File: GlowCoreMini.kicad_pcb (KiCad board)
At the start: 2 copper layers, 66 x 26.7 mm, 34 parts, among them J2 DC-042C-Z-2.5-A, J3 Conn_02x06_Counter_Clockwise, J4 WJ500V-5.08-3P, Q1 SK338P, Q2 MMBT2222A, Q3 MMBT2222A, SW1 TS-1185EC-C-D-B, U1 SN74AHCT32QPWRQ1, U2 ESP32-WROOM-32E (4MB), U3 BL1117-33CX, U4 CP2104

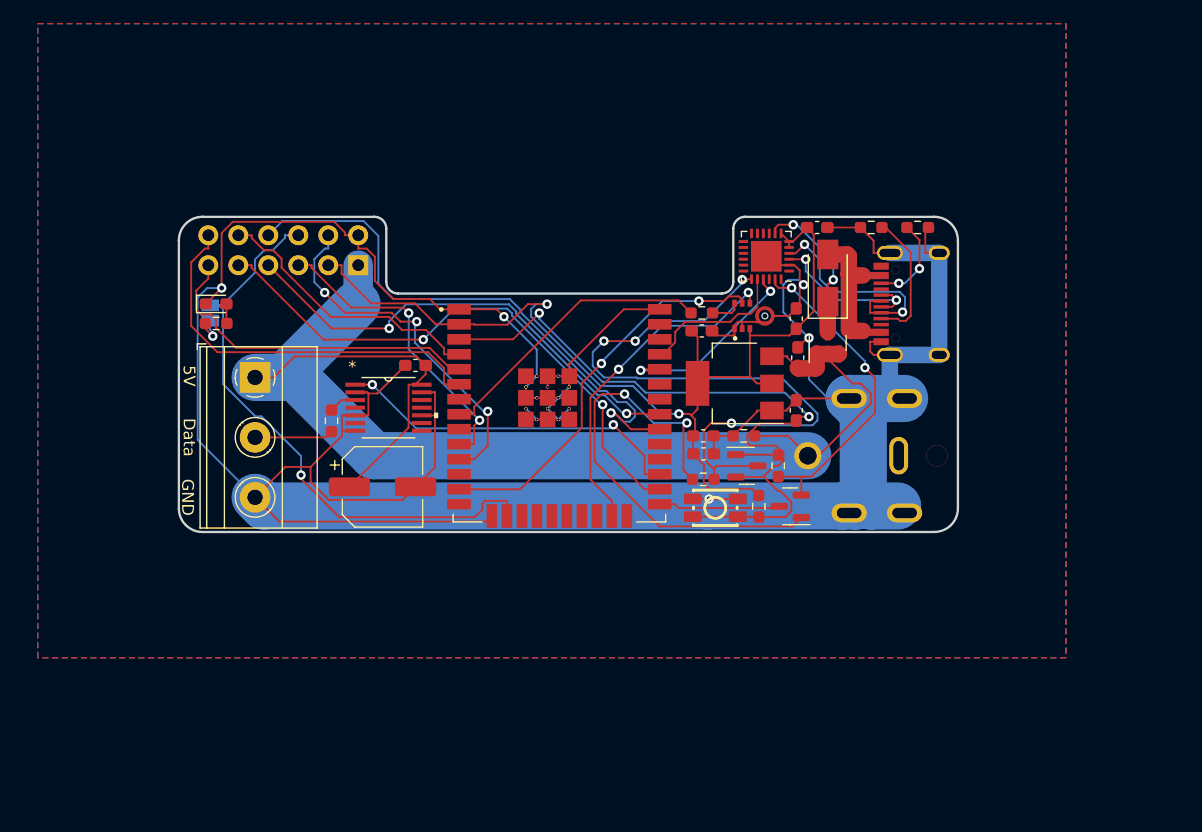
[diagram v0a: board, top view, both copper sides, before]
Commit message: updated pcb design (still in dev)
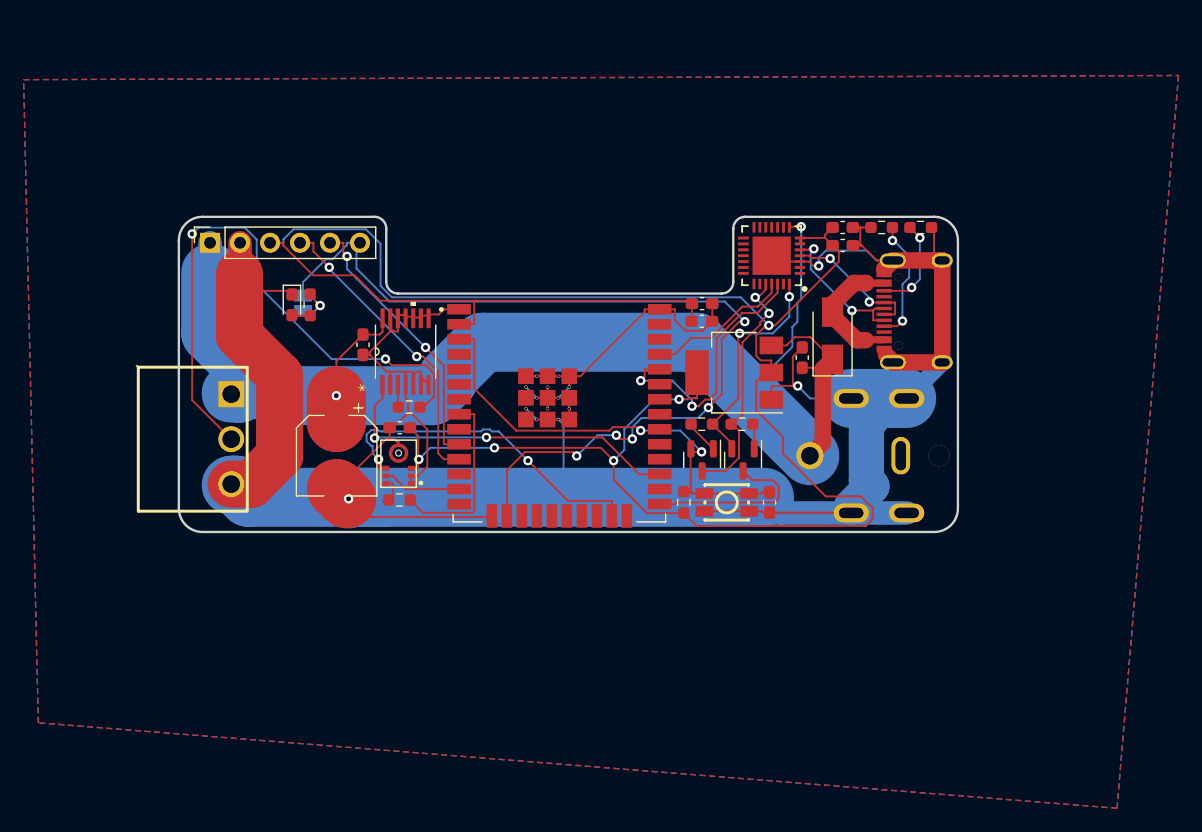
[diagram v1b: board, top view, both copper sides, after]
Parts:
- removed C5: 1uF, Capacitor_SMD:C_0603_1608Metric_Pad1.08x0.95mm_HandSolder
- removed J3: Conn_02x06_Counter_Clockwise, Connector_PinSocket_2.54mm:PinSocket_2x06_P2.54mm_Vertical
- removed J4: WJ500V-5.08-3P, TerminalBlock_Phoenix:TerminalBlock_Phoenix_MKDS-1,5-3-5.08_1x03_P5.08mm_Horizontal
- removed Q1: SK338P, Package_TO_SOT_SMD:SOT-23
- removed R2: 100K, Resistor_SMD:R_0603_1608Metric_Pad0.98x0.95mm_HandSolder
- added C10: 0.1uF, Capacitor_SMD:C_0603_1608Metric_Pad1.08x0.95mm_HandSolder, F.Cu at (163.3, 84.3)
- added J1: Conn_01x06, Connector_PinSocket_2.54mm:PinSocket_1x06_P2.54mm_Vertical, F.Cu at (109.7, 85.6)
- added P1: WJ15EDGRC-3.81-3P, WJ15EDGRC:WJ15EDGRC-3.81-3P, F.Cu at (108.3, 102.3)
- added logo: LOGO, LOGO, B.Cu at (146.1, 100.3)
- C6: value 10uF -> 4.7uF 6.3V 10%
- SW1: value TS-1185EC-C-D-B -> SW-SMD_4P-L3.7-W3.0-P1.50-LS4.7
- U1: value SN74AHCT32QPWRQ1 -> PW14
- U4: value CP2104 -> Val**; footprint Package_DFN_QFN:QFN-24-1EP_4x4mm_P0.5mm_EP2.6x2.6mm -> CP2102-GMR:CP2102-GMR
- moved C7 34.8 mm to (125.8, 101.3), turned to 0 degrees
- moved MK1 32.6 mm to (125.7, 104.3), turned to 180 degrees
- moved R4 30.1 mm to (125.8, 107.4), turned to 180 degrees
- moved C4 11.2 mm to (151.4, 92.3)
- moved R7 8.13 mm to (118.2, 90.9), turned to -90 degrees
- moved C9 8.12 mm to (157.1, 107.6), turned to 90 degrees
- moved Status_LED1 7.92 mm to (117.6, 90.8)
- moved R6 7.38 mm to (151.4, 101.0), turned to 180 degrees
- moved R1 6.68 mm to (126.6, 99.5), turned to 0 degrees
- moved D2 6.43 mm to (116.7, 90.9), turned to -90 degrees
- moved R8 6.36 mm to (149.9, 107.6), turned to -90 degrees
- moved R5 5.71 mm to (154.8, 101.0), turned to 0 degrees
- moved Q2 5.61 mm to (154.9, 104.0), turned to -90 degrees
- moved U1 4.97 mm to (126.3, 94.8), turned to 90 degrees
- moved D1 4.90 mm to (162.5, 93.5)
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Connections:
- C6 pad 1: +3V3 -> GND
- C6 pad 2: GND -> +3V3
- D1 pad 1: USB-C VBUS -> +5V
- U1 pad 11: unconnected-(U1-Pad11) -> GND
- U1 pad 12: unconnected-(U1-Pad12) -> GND
- U1 pad 4: unconnected-(U1-Pad4) -> GND
- U1 pad 6: unconnected-(U1-Pad6) -> GND
- U1 pad 8: unconnected-(U1-Pad8) -> GND
- U1 pad 9: unconnected-(U1-Pad9) -> GND
- U4 pad 19: RTS -> unconnected-(U4-Pad19)
- U4 pad 2: GND -> unconnected-(U4-Pad2)
- U4 pad 20: TXD0 -> unconnected-(U4-Pad20)
- U4 pad 21: RXD0 -> unconnected-(U4-Pad21)
- U4 pad 23: DTR -> unconnected-(U4-Pad23)
- U4 pad 24: unconnected-(U4-Pad24) -> RTS
- U4 pad 25: GND -> TXD0
- U4 pad 3: USB-C DATA+ -> GND
- U4 pad 4: USB-C DATA- -> USB-C DATA+
- U4 pad 5: +3V3 -> USB-C DATA-
- U4 pad 8: USB-C VBUS -> +5V
- USB1 pad B1A12: (no net) -> GND
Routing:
- net +3V3: track 87.7 -> 190.1 mm, vias 2 -> 5
- net IO18/MOSI: track 48.4 -> 0.00 mm, vias 1 -> 0
- net IO4/A5: track 48.1 -> 0.00 mm, vias 2 -> 0
- net Net-(R1-Pad2): track 6.68 -> 50.3 mm, vias 0 -> 2
- net IO19/MISO: track 40.6 -> 0.00 mm, vias 2 -> 0
- net Net-(Q2-Pad1): track 39.5 -> 2.14 mm, vias 2 -> 0
- net RTS: track 57.1 -> 20.9 mm, vias 4 -> 2
- net GND: track 317.3 -> 283.1 mm, vias 5 -> 3
- net I34/A2: track 34.0 -> 0.00 mm
- net I39/A3/SENSOR_VN: track 29.0 -> 0.00 mm
- net IO13: track 49.5 -> 77.5 mm, vias 1 -> 5
- net RESET: track 65.9 -> 39.1 mm
- net IO14/SCK: track 33.5 -> 6.67 mm, vias 2 -> 0
- net IO36/A4/SENSOR_VP: track 23.8 -> 0.00 mm
- net USB-C VBUS: track 13.0 -> 0.00 mm, vias 2 -> 0
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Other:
- board text added: "D"
- board text added: "DC: 5V, max 8A"
- board text added: "IO13 IO25 IO26 3.3V GND 5V"
- board text added: "Mini v1.0"
- board text added: "USB-C: 5V, max 3A"
- board text removed: "5V 3.3V IO25 IO19 IO4 IO39"
- board text removed: "Data"
- board text removed: "GND IO26 IO13 IO18 IO36 IO34"
- board text removed: "USB-C power -> 5V, up to 3A DC power -> 5V, up to 8A"

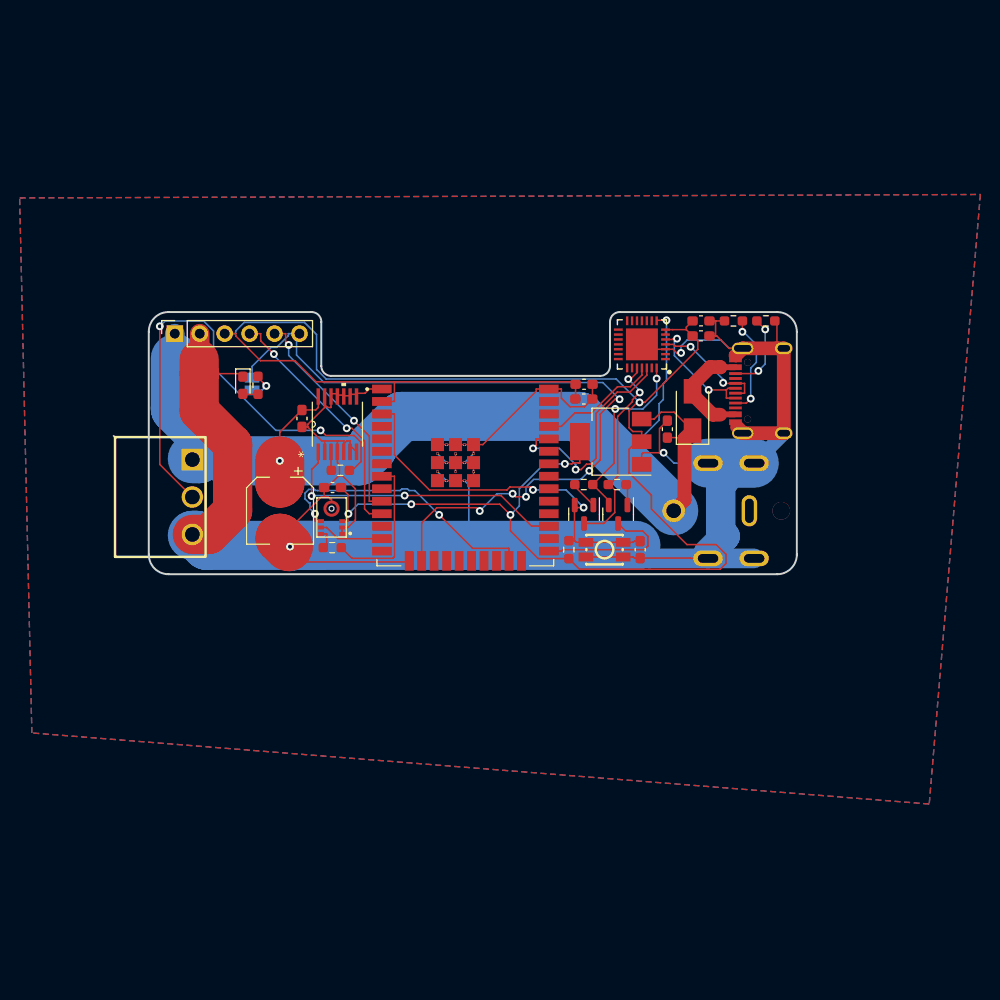
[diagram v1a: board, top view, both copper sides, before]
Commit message: last fixes to prototype v1
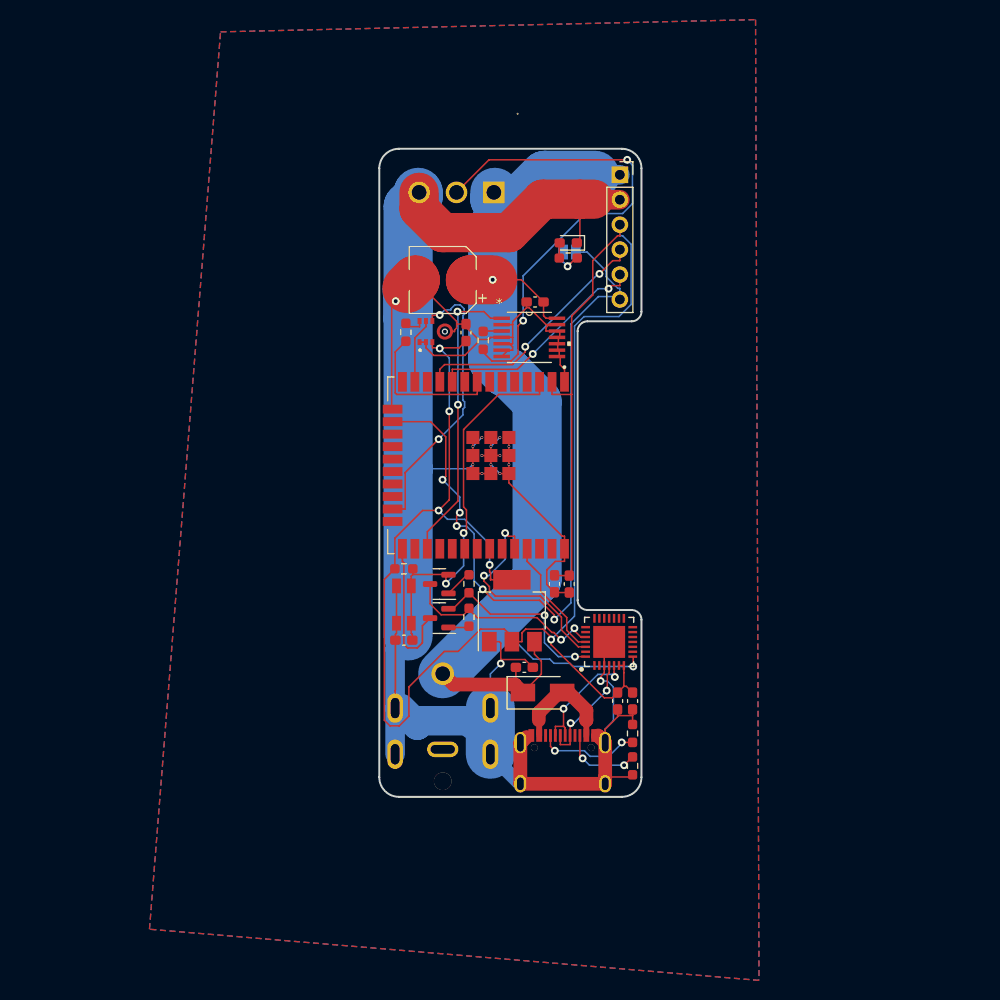
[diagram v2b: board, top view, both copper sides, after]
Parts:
- moved J1 48.1 mm to (155.1, 69.4), turned to 0 degrees
- moved R9 47.3 mm to (156.4, 129.6), turned to 90 degrees
- moved P1 45.7 mm to (138.4, 68.0), turned to 180 degrees
- moved R3 43.2 mm to (156.4, 126.3), turned to -90 degrees
- moved USB1 42.6 mm to (149.2, 129.0), turned to 0 degrees
- moved C10 39.3 mm to (156.4, 123.0), turned to -90 degrees
- moved C6 38.1 mm to (154.8, 123.0), turned to 90 degrees
- moved D2 36.2 mm to (149.8, 76.4), turned to 180 degrees
- moved Status_LED1 35.0 mm to (149.9, 77.3), turned to 180 degrees
- moved J2 34.5 mm to (137.0, 124.4), turned to 90 degrees
- moved R7 34.1 mm to (149.8, 77.9), turned to 180 degrees
- moved D1 32.5 mm to (147.2, 122.2), turned to 0 degrees
- moved U4 30.5 mm to (154.0, 117.0), turned to 90 degrees
- moved C2 28.8 mm to (137.0, 80.2), turned to 180 degrees
- moved C3 28.3 mm to (145.3, 119.6), turned to 180 degrees
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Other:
- board size 66 x 26.7 mm -> 26.7 x 66 mm
- board text added: "5V (8A max!) GND 3.3V IO26 IO25 IO13"
- board text removed: "IO13 IO25 IO26 3.3V GND 5V"

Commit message: update design
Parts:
- removed logo: LOGO, LOGO
- added C11: 220uF 10V, Capacitor_SMD:CP_Elec_6.3x5.4, F.Cu at (147.4, 128.3)
- added C12: 220uF 10V, Capacitor_SMD:CP_Elec_6.3x5.4, F.Cu at (137.6, 121.1)
- added C5: 220uF 10V, Capacitor_SMD:CP_Elec_6.3x5.4, F.Cu at (147.3, 121.1)
- added F1: BSMD1812-300-16V, Fuse:Fuse_1812_4532Metric_Pad1.30x3.40mm_HandSolder, F.Cu at (150.1, 137.5)
- added F2: JK16-800, JK16-800:JK16-800, F.Cu at (139.9, 134.6)
- added G***: LOGO, LOGO, B.Cu at (155.4, 135.1)
- added G***: LOGO, LOGO, B.Cu at (145.2, 105.2)
- added REF**: OSHW-Logo2_7.3x6mm_SilkScreen, Symbol:OSHW-Logo2_7.3x6mm_SilkScreen, B.Cu at (146.6, 134.9)
- C2: value 220uF 10V 6.3x5.4mm -> 220uF 10V
- moved C2 48.1 mm to (137.6, 128.2)
- moved D2 35.9 mm to (158.4, 111.2)
- moved R7 35.9 mm to (158.4, 112.7)
- moved Status_LED1 35.6 mm to (158.3, 111.9)
- moved R3 22.2 mm to (159.5, 148.4), turned to 90 degrees
- moved R9 18.8 mm to (158.0, 148.4)
- moved J2 17.6 mm to (139.3, 141.8)
- moved USB1 17.0 mm to (151.5, 145.9)
- moved R4 15.7 mm to (146.5, 76.9), turned to 0 degrees
- moved C3 13.2 mm to (143.7, 106.5)
- moved Q2 13.0 mm to (149.7, 115.4), turned to -90 degrees
- moved C4 12.4 mm to (136.9, 106.7), turned to 180 degrees
- moved D1 12.0 mm to (150.4, 133.8)
- moved MK1 11.6 mm to (146.5, 80.0), turned to 0 degrees
- moved U4 11.0 mm to (157.0, 127.6)
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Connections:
- net IO12 renamed IO12/MISO
- net IO18/MOSI renamed IO18
- net IO19/MISO renamed IO19
- J2 pad 3: +5V -> Net-(F2-Pad2)
- U2 pad 16: IO13 -> IO13/MOSI
- USB1 pad A4B9: Net-(D1-Pad2) -> Net-(F1-Pad1)
- USB1 pad B4A9: Net-(D1-Pad2) -> Net-(F1-Pad1)
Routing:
- net GND: track 283.1 -> 419.4 mm, vias 3 -> 7
- net +3V3: track 190.1 -> 136.1 mm, vias 5 -> 2
- net +5V: track 114.6 -> 154.0 mm, vias 2 -> 6
- net IO13: track 77.5 -> 43.1 mm, vias 5 -> 0
- net Net-(P1-Pad2): track 50.3 -> 23.0 mm, vias 2 -> 0
- net Net-(F1-Pad1): track 0.00 -> 16.5 mm
- net IO14/SCK: track 6.67 -> 21.7 mm
- net TXD0: track 12.4 -> 27.0 mm
- net RESET: track 39.1 -> 49.5 mm
- net USB-C DATA+: track 11.8 -> 20.9 mm
- net IO0: track 14.9 -> 23.7 mm
- net Net-(D1-Pad2): track 11.6 -> 3.81 mm
- net DTR: track 19.0 -> 26.8 mm
- net USB-C DATA-: track 12.6 -> 19.3 mm
- net Net-(F2-Pad2): track 0.00 -> 5.93 mm
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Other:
- board size 26.7 x 66 mm -> 31 x 89.1 mm
- board text added: "5V D GND"
- board text added: "5V GND 3.3V IO26 IO25 IO13"
- board text added: "GlowCore Mini"
- board text added: "PCB files: https://bit.ly/3JLodEJ"
- board text added: "designed by"
- board text added: "v1.1"
- board text removed: "5V"
- board text removed: "5V (8A max!) GND 3.3V IO26 IO25 IO13"
- board text removed: "D"
- board text removed: "GND"
- board text removed: "Mini v1.0"

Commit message: work on updated pcb design
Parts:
- removed C11, C12: 220uF 10V, Capacitor_SMD:CP_Elec_6.3x5.4
- removed F1: BSMD1812-300-16V, Fuse:Fuse_1812_4532Metric_Pad1.30x3.40mm_HandSolder
- removed F2: JK16-800, JK16-800:JK16-800
- removed R4: 100K, Resistor_SMD:R_0603_1608Metric_Pad0.98x0.95mm_HandSolder
- removed Status_LED1: SolderJumper_2_Open, Jumper:SolderJumper-2_P1.3mm_Open_Pad1.0x1.5mm
- added R2: 100K, Resistor_SMD:R_0603_1608Metric_Pad0.98x0.95mm_HandSolder, F.Cu at (146.5, 87.5)
- D1: value B340A-13-F -> SS54
- SW1: value SW-SMD_4P-L3.7-W3.0-P1.50-LS4.7 -> TS-1185EC-C-D-B
- U1: value PW14 -> SN74AHCT32QPWRQ1
- U4: value Val** -> CP2102-GMR
- moved REF** 49.2 mm to (138.3, 86.3)
- moved G*** 49.0 mm to (147.8, 86.7)
- moved C5 39.2 mm to (138.3, 82.9), turned to 180 degrees
- moved R8 21.4 mm to (135.7, 128.6), turned to -90 degrees
- moved SW1 18.7 mm to (139.4, 128.6), turned to 180 degrees
- moved G*** 18.2 mm to (145.9, 123.4)
- moved C9 17.2 mm to (143.0, 128.6), turned to 90 degrees
- moved D2 10.5 mm to (158.4, 121.7)
- moved C1 10.5 mm to (139.6, 87.5)
- moved C3 10.5 mm to (143.7, 117.0)
- moved C4 10.5 mm to (136.9, 117.2)
- moved C7 10.5 mm to (146.4, 93.6)
- moved C8 10.5 mm to (140.3, 117.1)
- moved J1 10.5 mm to (158.2, 75.1)
- moved MK1 10.5 mm to (146.5, 90.5)
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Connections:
- J2 pad 3: Net-(F2-Pad2) -> +5V
- MK1 pad 7: Net-(MK1-Pad7) -> IO32/SD
- R7 pad 1: Net-(R7-Pad1) -> IO13
- USB1 pad A4B9: Net-(F1-Pad1) -> Net-(D1-Pad2)
- USB1 pad B4A9: Net-(F1-Pad1) -> Net-(D1-Pad2)
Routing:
- net GND: track 419.4 -> 0.00 mm, vias 7 -> 0
- net +5V: track 154.0 -> 0.00 mm, vias 6 -> 0
- net +3V3: track 136.1 -> 0.00 mm, vias 2 -> 0
- net RESET: track 49.5 -> 0.00 mm, vias 2 -> 0
- net IO13: track 43.1 -> 0.00 mm
- net IO16/LED1: track 31.5 -> 0.00 mm
- net IO15/WS: track 30.3 -> 0.00 mm, vias 2 -> 0
- net RXD0: track 28.2 -> 0.00 mm
- net TXD0: track 27.0 -> 0.00 mm
- net DTR: track 26.8 -> 0.00 mm, vias 2 -> 0
- net IO26/A0/DAC2: track 25.9 -> 0.00 mm, vias 1 -> 0
- net IO0: track 23.7 -> 0.00 mm
- net IO25/A1/DAC1: track 23.4 -> 0.00 mm, vias 1 -> 0
- net Net-(P1-Pad2): track 23.0 -> 0.00 mm
- net RTS: track 22.7 -> 0.00 mm, vias 2 -> 0
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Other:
- board size 31 x 89.1 mm -> 28 x 77.3 mm
- board text added: "GND D 5V"
- board text removed: "Status LED"
